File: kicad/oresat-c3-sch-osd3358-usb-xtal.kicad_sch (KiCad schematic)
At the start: 36 parts, among them U1 OSD3358-512M-BSM, U11 RCLAMP0504FB, Y1 ECS-240-12-30BQ-AEN-TR, Y2 ABS07-32.768KHZ-T

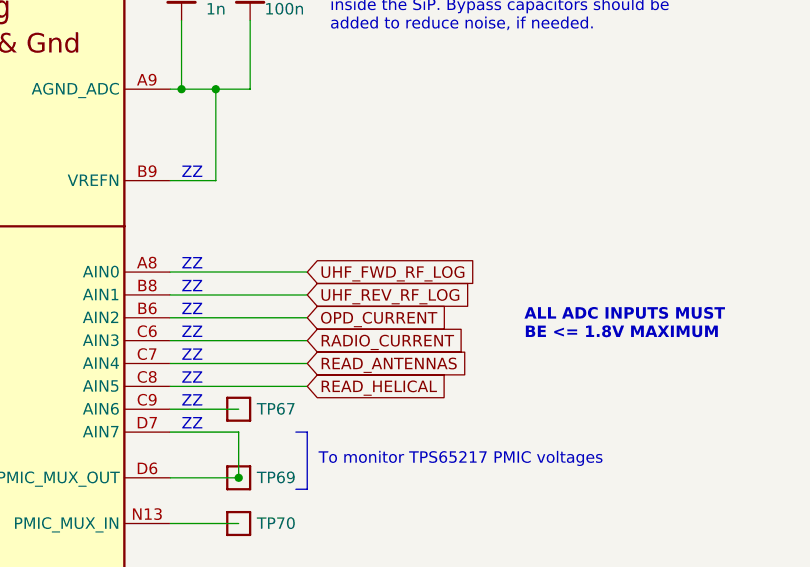
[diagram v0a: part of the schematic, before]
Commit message: Removed UF band
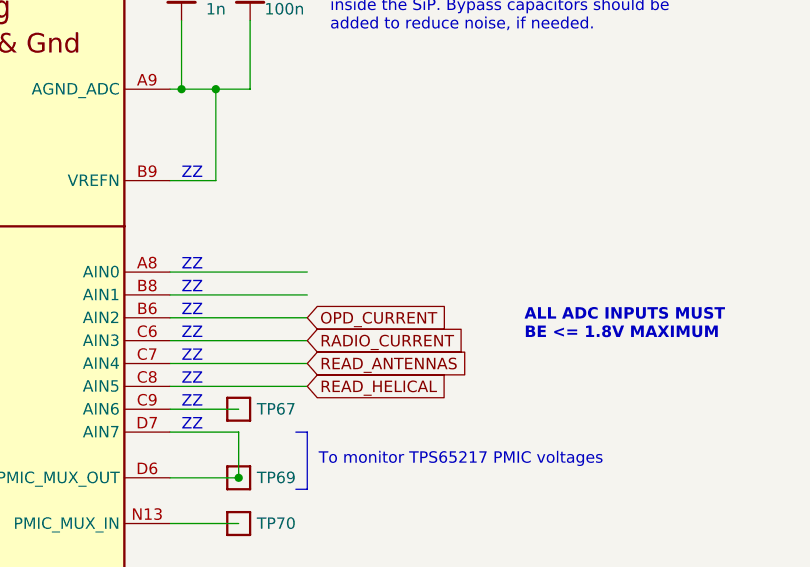
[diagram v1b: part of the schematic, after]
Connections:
- net UHF_FWD_RF_LOG: no longer names the net of U1.A8 (AIN0)
- net UHF_REV_RF_LOG: no longer names the net of U1.B8 (AIN1)
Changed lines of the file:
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@@
-    )
-  )
-  (global_label "UHF_FWD_RF_LOG" (shape input) (at 271.78 121.92 0) (fields_autoplaced)
-    (effects (font (size 1.27 1.27)) (justify left))
-    (property "Intersheetrefs" "${INTERSHEET_REFS}" (at 291.1354 121.92 0)
-      (effects (font (size 1.27 1.27)) (justify left))
     )
   )
@@
       (effects (font (size 1.27 1.27)) (justify left))
     )
-  )
-  (global_label "UHF_REV_RF_LOG" (shape input) (at 271.78 124.46 0) (fields_autoplaced)
-    (effects (font (size 1.27 1.27)) (justify left))
-    (property "Intersheetrefs" "${INTERSHEET_REFS}" (at 290.833 124.46 0)
-      (effects (font (size 1.27 1.27)) (justify left))
-    )

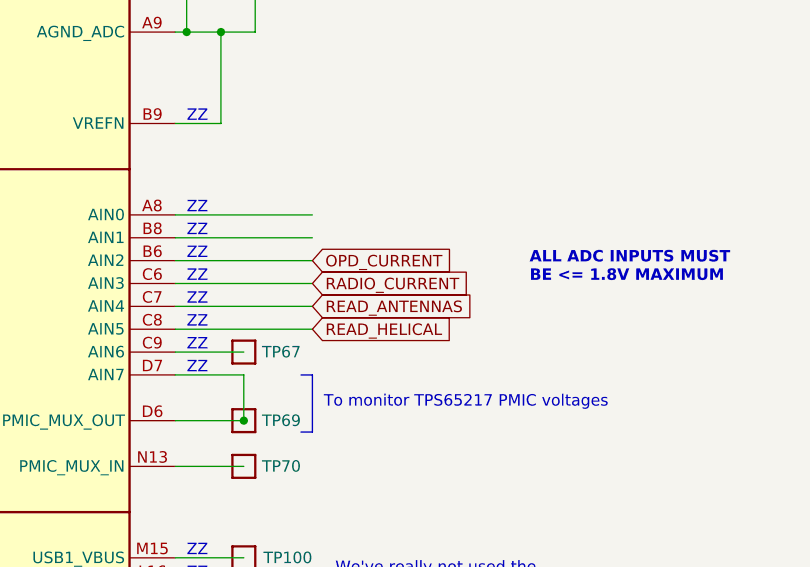
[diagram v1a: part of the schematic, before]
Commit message: Removed power switching circuitry
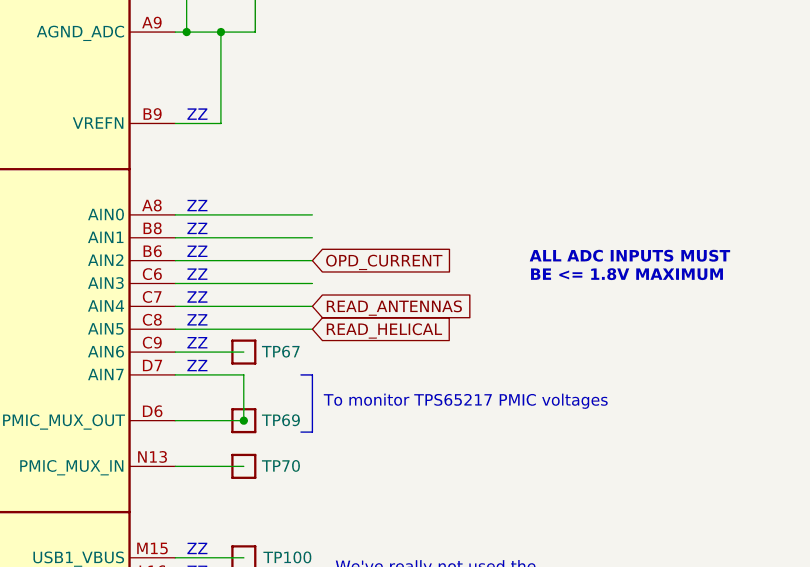
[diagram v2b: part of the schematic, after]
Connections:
- net RADIO_CURRENT: no longer names the net of U1.C6 (AIN3)
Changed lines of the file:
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@@
-    )
-  )
-  (global_label "RADIO_CURRENT" (shape input) (at 271.78 129.54 0) (fields_autoplaced)
-    (effects (font (size 1.27 1.27)) (justify left))
-    (property "Intersheetrefs" "${INTERSHEET_REFS}" (at 289.8049 129.54 0)
-      (effects (font (size 1.27 1.27)) (justify left))
     )
   )

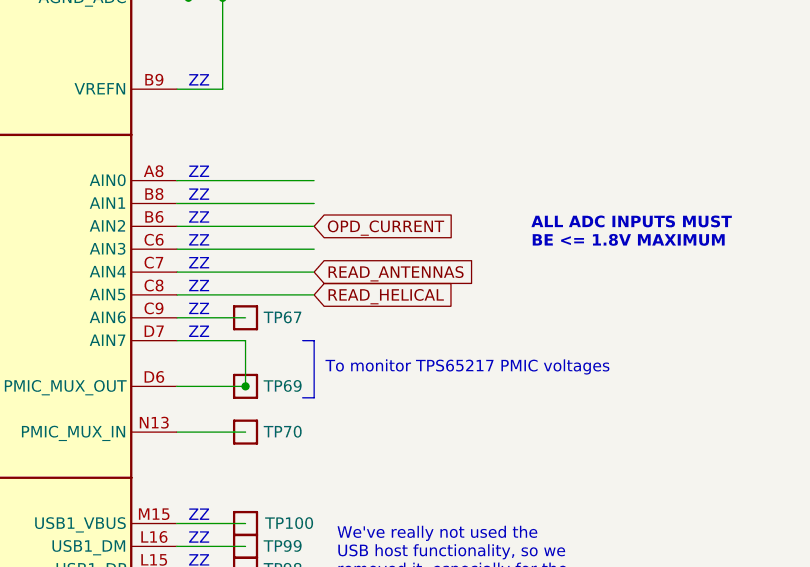
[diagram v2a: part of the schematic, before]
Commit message: Removed antenna deployers, fixed
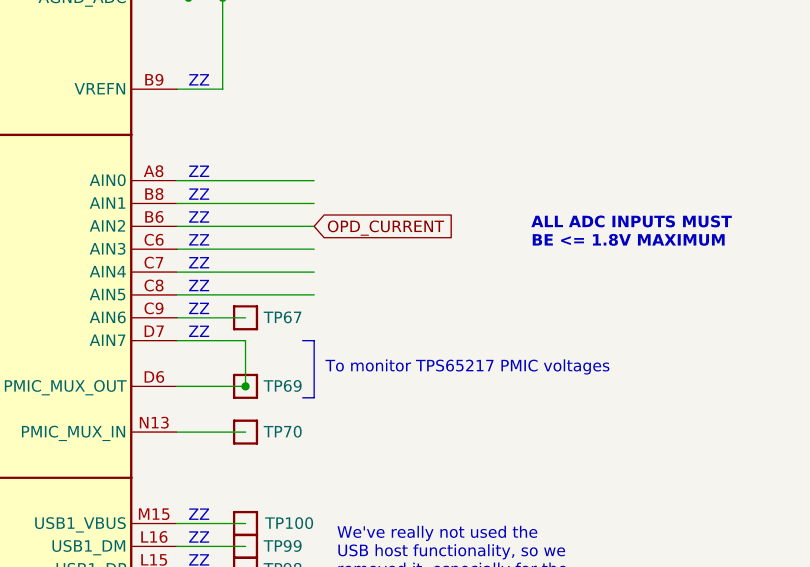
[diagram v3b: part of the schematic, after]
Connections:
- net READ_ANTENNAS: no longer names the net of U1.C7 (AIN4)
- net READ_HELICAL: no longer names the net of U1.C8 (AIN5)
